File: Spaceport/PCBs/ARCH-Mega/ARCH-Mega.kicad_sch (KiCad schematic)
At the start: 69 parts, among them J1 Conn_01x04_Pin, J2 Conn_01x05_Pin, U1 STM32C011F6U6TR, U2 TPS51388VABR, U3 LDL212PVR, U4 NPS3005BGPZ, U5 NPS3005BGPZ, U6 NPS3005BGPZ, U7 NPS3005BGPZ, U8 NPS3005BGPZ, U9 NPS3005BGPZ

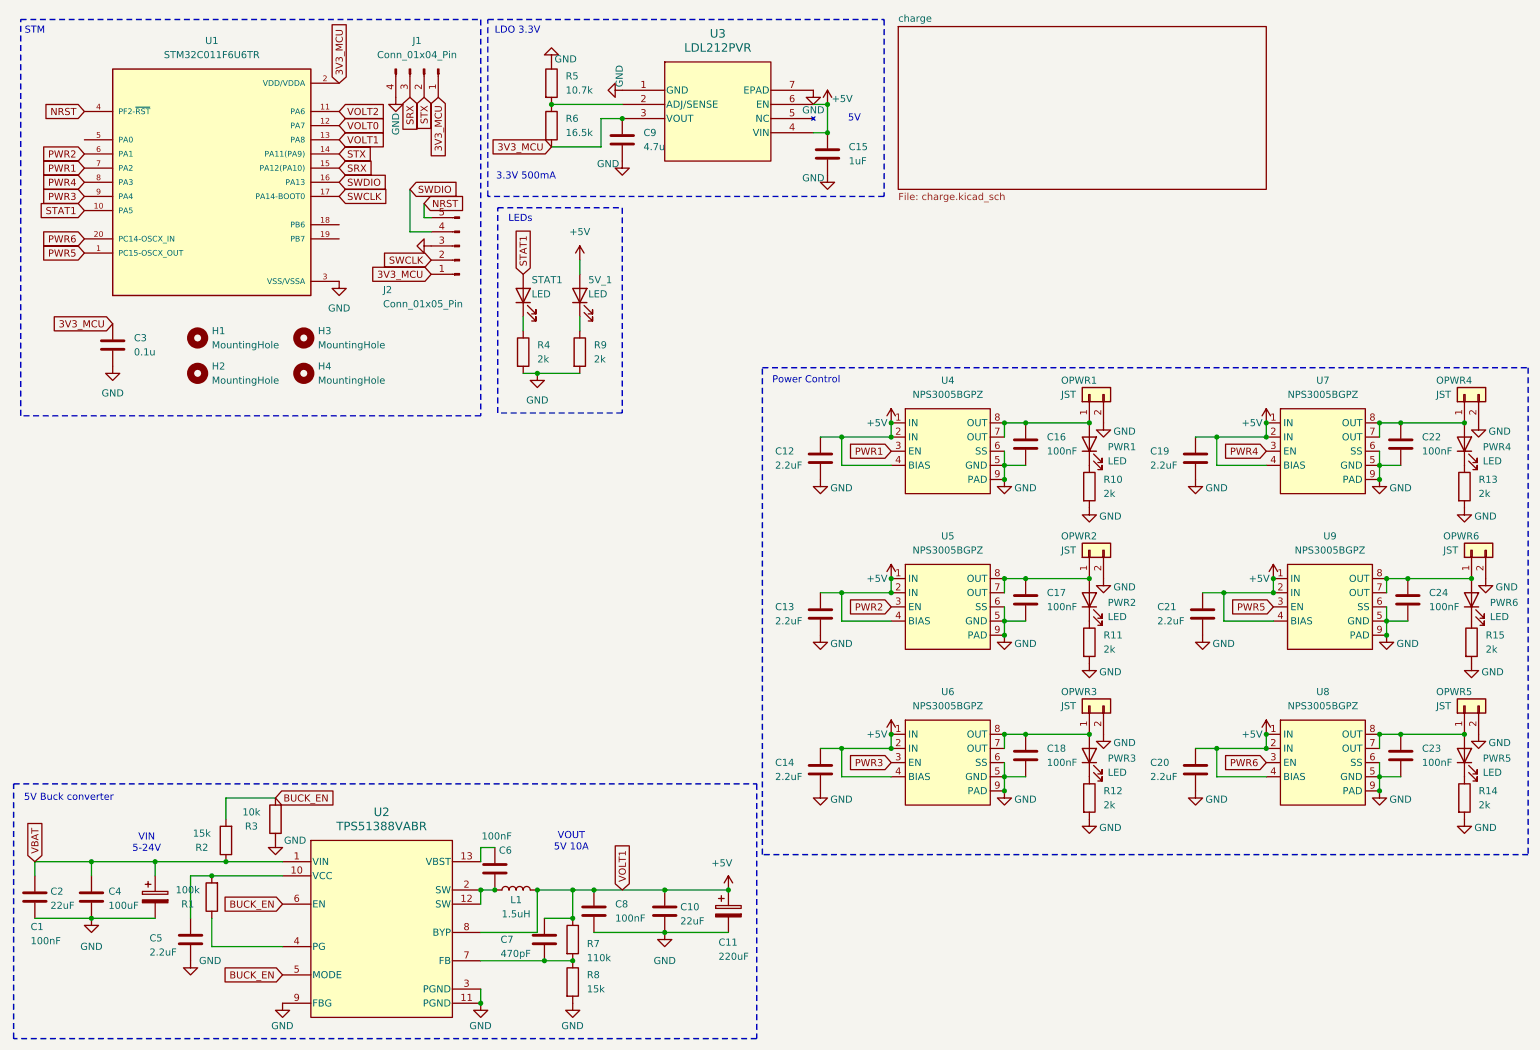
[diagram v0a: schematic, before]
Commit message: Final ARCH-Mega
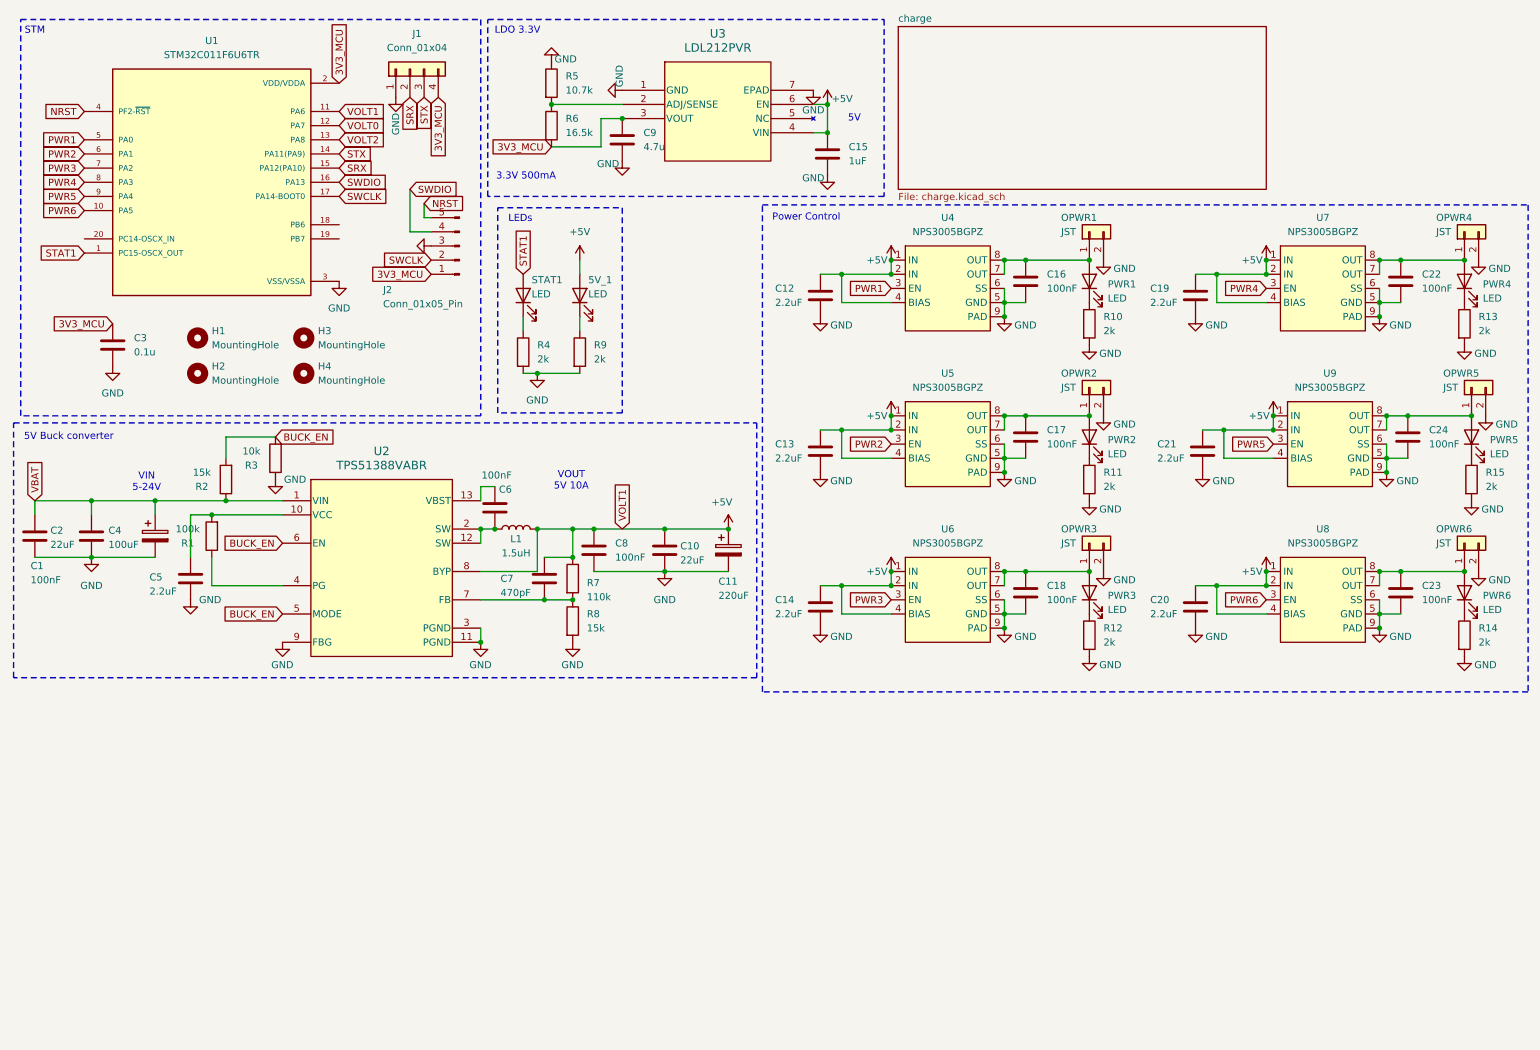
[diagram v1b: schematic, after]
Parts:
- removed J1: Conn_01x04_Pin, Avionics:JST_XH_1x4_P2.50mm_Horizontal_Small, symbol Connector:Conn_01x04_Pin
- added J1: Conn_01x04, Avionics:JST_XH_1x4_P2.50mm_Horizontal_Small, symbol Connector_Generic:Conn_01x04
- C5: footprint Capacitor_SMD:C_0805_2012Metric -> Capacitor_SMD:C_0603_1608Metric
- renumbered OPWR6 to OPWR5, OPWR5 to OPWR6, PWR6 to PWR5, PWR5 to PWR6
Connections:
- net +5V: now also U1.11 (PA6); no longer U1.13 (PA8)
- net 3V3_MCU: now also J1.4 (Pin_4)
- net GND: now also J1.1 (Pin_1)
- net PWR1: now also U1.5 (PA0); no longer U1.7 (PA2)
- net PWR3: now also U1.7 (PA2); no longer U1.9 (PA4)
- net PWR5: now also U1.9 (PA4); no longer U1.1 (PC15-OSCX_OUT)
- net PWR6: now also U1.10 (PA5); no longer U1.20 (PC14-OSCX_IN)
- net SRX: now also J1.2 (Pin_2)
- net STAT1: now also U1.1 (PC15-OSCX_OUT); no longer U1.10 (PA5)
- net STX: now also J1.3 (Pin_3)
- net VOLT2: now also U1.13 (PA8); no longer U1.11 (PA6)
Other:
- moved on the sheet: C1, C10, C11, C12, C13, C14, C16, C17, C18, C19, C2, C20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

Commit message: Most schematic fixes for ARCH-Mega
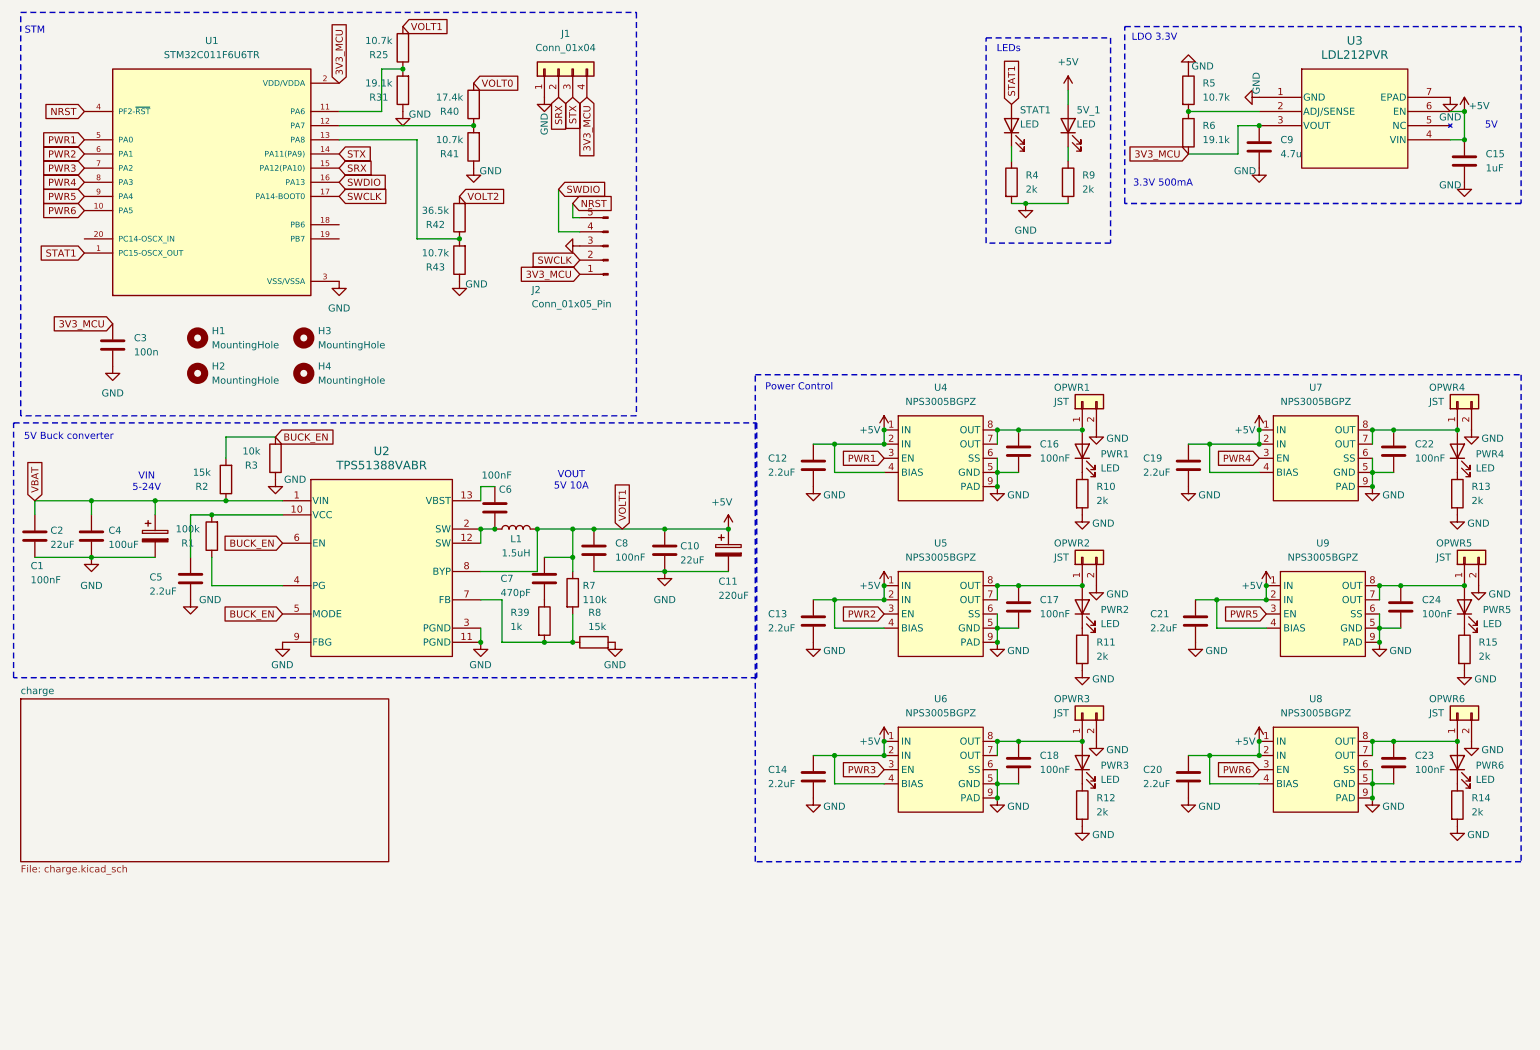
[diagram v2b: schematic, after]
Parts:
- added R25, R41, R43: 10.7k, Resistor_SMD:R_0603_1608Metric, symbol Device:R
- added R31: 19.1k, Resistor_SMD:R_0603_1608Metric, symbol Device:R
- added R39: 1k, Resistor_SMD:R_0603_1608Metric, symbol Device:R
- added R40: 17.4k, Resistor_SMD:R_0603_1608Metric, symbol Device:R
- added R42: 36.5k, Resistor_SMD:R_0603_1608Metric, symbol Device:R
- C3: value 0.1u -> 100n
- R6: value 16.5k -> 19.1k
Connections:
- net +5V: now also R25.2; no longer U1.11 (PA6)
- net GND: now also R31.1, R41.1, R43.1
- net VOLT0: now also R40.2; no longer U1.12 (PA7)
- net VOLT2: now also R42.2; no longer U1.13 (PA8)
- net at R7.2, R8.1, U2.7 (FB): now also R39.2; no longer C7.2
- new net: R42.1, R43.2, U1.13 (PA8)
- new net: R25.1, R31.2, U1.11 (PA6)
- new net: R40.1, R41.2, U1.12 (PA7)
- new net: C7.2, R39.1
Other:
- moved on the sheet: 5V_1, C12, C13, C14, C15, C16, C17, C18, C19, C20, C21, C22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
